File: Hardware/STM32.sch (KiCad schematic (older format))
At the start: 3 parts

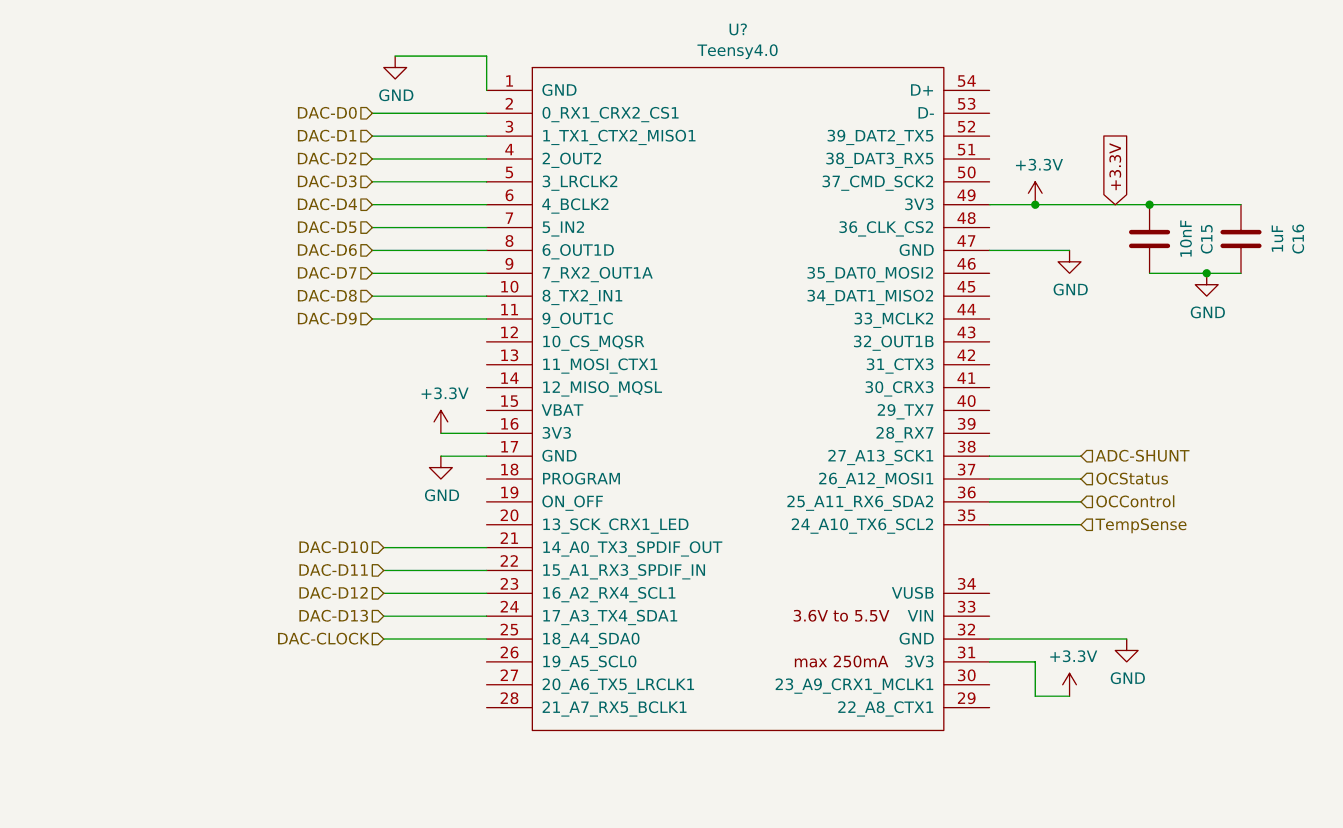
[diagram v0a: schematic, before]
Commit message: external ADC added
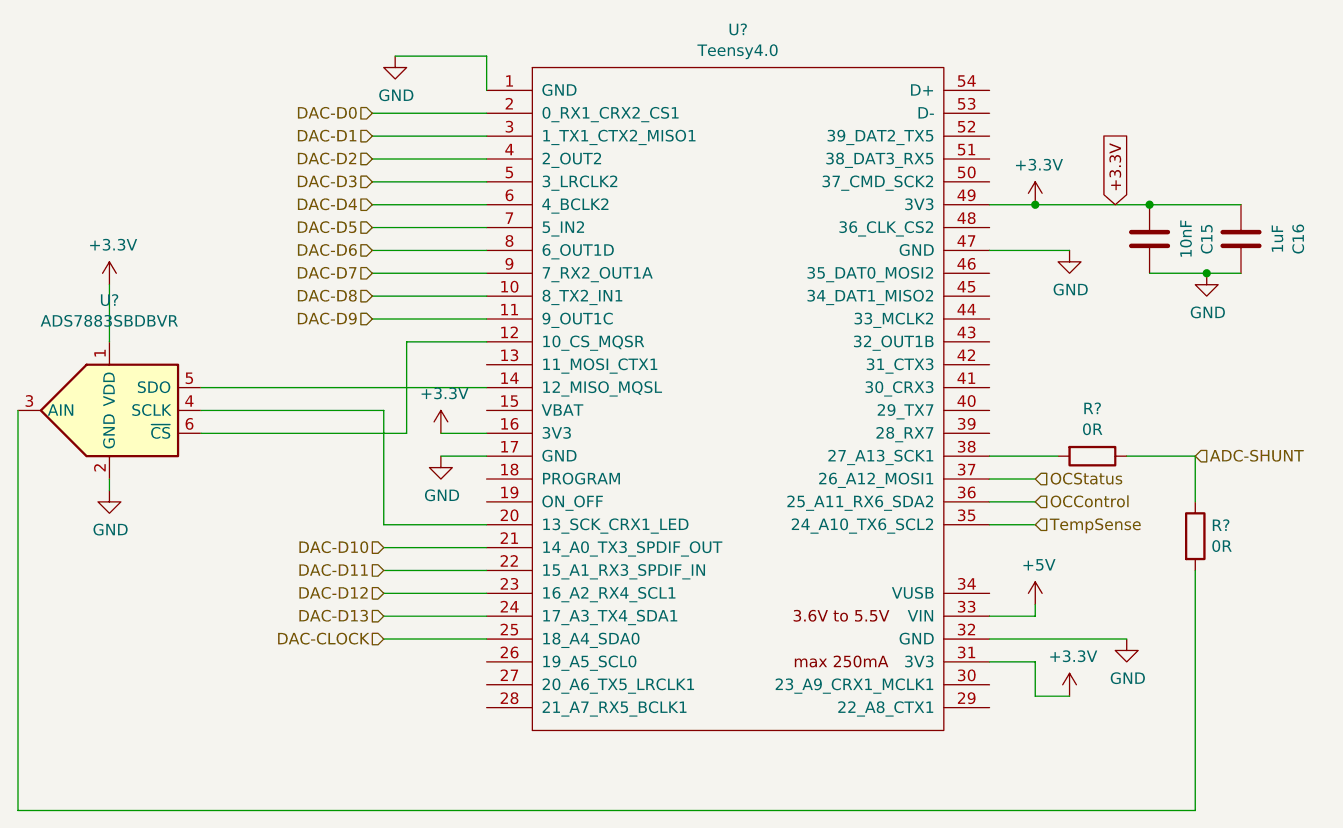
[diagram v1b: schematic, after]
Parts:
- added R? (x2): 0R, symbol Device:R
- added U?: ADS7883SBDBVR, Package_TO_SOT_SMD:TSOT-23-6, symbol Analog_ADC:ADS7866
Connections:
- net +3V3: now also U?.1 (VDD)
- net ADC-SHUNT: now also R?.1, R?.1; no longer U?.38 (27_A13_SCK1)
- net GND: now also U?.2 (GND)
- net at U?.12 (10_CS_MQSR): now also U?.6 (~CS)
- net at U?.14 (12_MISO_MQSL): now also U?.5 (SDO)
- net at U?.20 (13_SCK_CRX1_LED): now also U?.4 (SCLK)
- net +5V: now reaches U?.33 (VIN)
- new net: R?.2, U?.38 (27_A13_SCK1)
- new net: R?.2, U?.3 (AIN)
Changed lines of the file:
@@
 DAC-CLOCK
 Wire Wire Line
-	7350 3900 6950 3900
-Wire Wire Line
-	6950 4000 7350 4000
-Wire Wire Line
-	7350 4200 6950 4200
+	6950 4000 7150 4000
+Wire Wire Line
+	7150 4200 6950 4200
 $Comp
 L teensy:Teensy4.0 U?
@@
 Wire Wire Line
 	4300 4700 4750 4700
-Text HLabel 7350 4200 2    50   Input ~ 0
+Text HLabel 7150 4200 2    50   Input ~ 0
 TempSense
-Text HLabel 7350 4000 2    50   Input ~ 0
-OCStatus
-Text HLabel 7350 3900 2    50   Input ~ 0
+Text HLabel 7850 3900 2    50   Input ~ 0
 ADC-SHUNT
 Wire Wire Line
-	6950 4100 7350 4100
-Text HLabel 7350 4100 2    50   Input ~ 0
-OCControl
+	6950 4100 7150 4100
 $Comp
 L power:+3.3V #PWR?
@@
 Wire Wire Line
 	7150 2800 7650 2800
+$Comp
+L Analog_ADC:ADS7866 U?
+U 1 1 5FCB3601
+P 3100 3700
+F 0 "U?" H 3100 4181 50  0000 C CNN
+F 1 "ADS7883SBDBVR" H 3100 4090 50  0000 C CNN
+F 2 "Package_TO_SOT_SMD:TSOT-23-6" H 3100 3650 50  0001 C CNN
+F 3 "http://www.ti.com/lit/ds/symlink/ads7866.pdf" H 3150 3950 50  0001 C CNN
+	1    3100 3700
+	1    0    0    -1
+$EndComp
+Wire Wire Line
+	2700 3700 2700 5450
+Wire Wire Line
+	2700 5450 7850 5450
+Wire Wire Line
+	6950 3900 7250 3900
+Text HLabel 7150 4100 2    50   Input ~ 0
+OCControl
+Text HLabel 7150 4000 2    50   Input ~ 0
+OCStatus
+$Comp
+L power:+5V #PWR?
+U 1 1 5FCBF530
+P 7150 4550
+F 0 "#PWR?" H 7150 4400 50  0001 C CNN
+F 1 "+5V" H 7165 4723 50  0000 C CNN
+F 2 "" H 7150 4550 50  0001 C CNN
+F 3 "" H 7150 4550 50  0001 C CNN
+	1    7150 4550
+	1    0    0    -1
+$EndComp
+Wire Wire Line
+	6950 4600 7150 4600
+Wire Wire Line
+	7150 4600 7150 4550
+Wire Wire Line
+	4300 4200 4750 4200
+Wire Wire Line
+	3500 3700 4300 3700
+Wire Wire Line
+	4300 3700 4300 4200
+Wire Wire Line
+	3500 3800 4400 3800
+Wire Wire Line
+	4400 3800 4400 3400
+Wire Wire Line
+	4400 3400 4750 3400
+Wire Wire Line
+	3500 3600 4750 3600
+$Comp
+L power:+3.3V #PWR?
+U 1 1 5FCCE399
+P 3100 3150
+F 0 "#PWR?" H 3100 3000 50  0001 C CNN
+F 1 "+3.3V" H 3115 3323 50  0000 C CNN
+F 2 "" H 3100 3150 50  0001 C CNN
+F 3 "" H 3100 3150 50  0001 C CNN
+	1    3100 3150
+	1    0    0    -1
+$EndComp
+$Comp
+L power:GND #PWR?
+U 1 1 5FCCE9B3
+P 3100 4050
+F 0 "#PWR?" H 3100 3800 50  0001 C CNN
+F 1 "GND" H 3105 3877 50  0000 C CNN
+F 2 "" H 3100 4050 50  0001 C CNN
+F 3 "" H 3100 4050 50  0001 C CNN
+	1    3100 4050
+	1    0    0    -1
+$EndComp
+Wire Wire Line
+	3100 4050 3100 4000
+Wire Wire Line
+	3100 3400 3100 3150
+Wire Wire Line
+	7850 5450 7850 4400
+$Comp
+L Device:R R?
+U 1 1 5FCD541A
+P 7850 4250
+F 0 "R?" H 7920 4296 50  0000 L CNN
+F 1 "0R" H 7920 4205 50  0000 L CNN
+F 2 "" V 7780 4250 50  0001 C CNN
+F 3 "~" H 7850 4250 50  0001 C CNN
+	1    7850 4250
+	1    0    0    -1
+$EndComp
+$Comp
+L Device:R R?
+U 1 1 5FCD592E
+P 7400 3900
+F 0 "R?" V 7193 3900 50  0000 C CNN
+F 1 "0R" V 7284 3900 50  0000 C CNN
+F 2 "" V 7330 3900 50  0001 C CNN
+F 3 "~" H 7400 3900 50  0001 C CNN
+	1    7400 3900
+	0    1    1    0
+$EndComp
+Wire Wire Line
+	7550 3900 7850 3900
+Wire Wire Line
+	7850 4100 7850 3900
 $EndSCHEMATC

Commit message: project import to kicad 5.1.
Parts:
- U?: symbol teensy:Teensy4.0 -> Laser-Driver-v3-rescue:Teensy4.0-teensy
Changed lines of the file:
@@
 EESchema Schematic File Version 4
-LIBS:Laser-Driver-v3-cache
-EELAYER 29 0
+EELAYER 30 0
 EELAYER END
 $Descr A4 11693 8268
@@
 	7150 4200 6950 4200
 $Comp
-L teensy:Teensy4.0 U?
+L Laser-Driver-v3-rescue:Teensy4.0-teensy U?
 U 1 1 5F63D3E1
 P 5850 3650
+AR Path="/5F63D3E1" Ref="U?"  Part="1"
+AR Path="/5D037190/5F63D3E1" Ref="U?"  Part="1"
 F 0 "U?" H 5850 5265 50  0000 C CNN
 F 1 "Teensy4.0" H 5850 5174 50  0000 C CNN
